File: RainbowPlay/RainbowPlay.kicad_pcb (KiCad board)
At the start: 2 copper layers, 140 x 80 mm, 23 parts, among them J1 GPIO_CONNECTOR, J2 PJ-102A, U1 LM386, U2 LM386

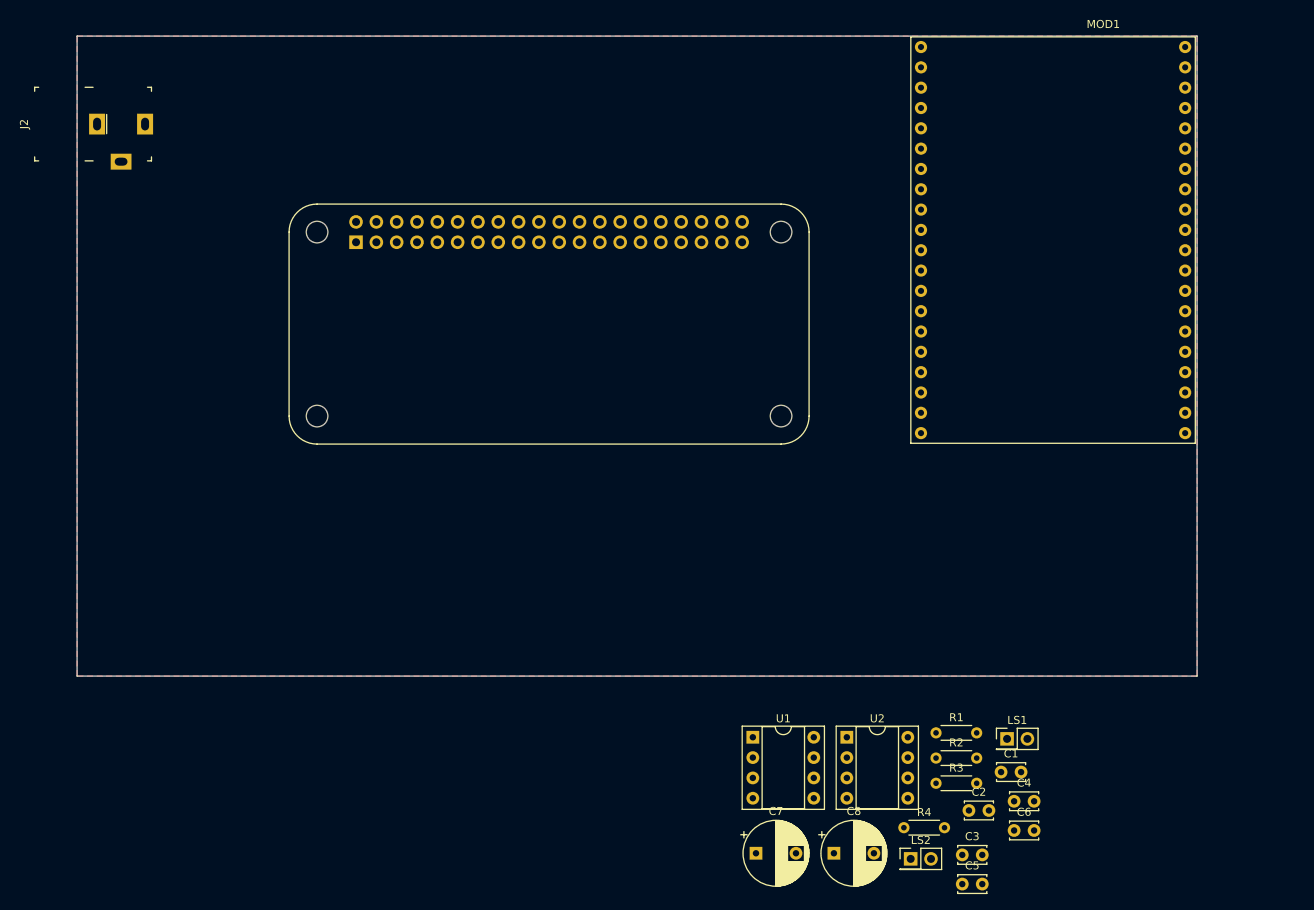
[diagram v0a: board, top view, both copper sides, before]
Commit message: Initial development in progress
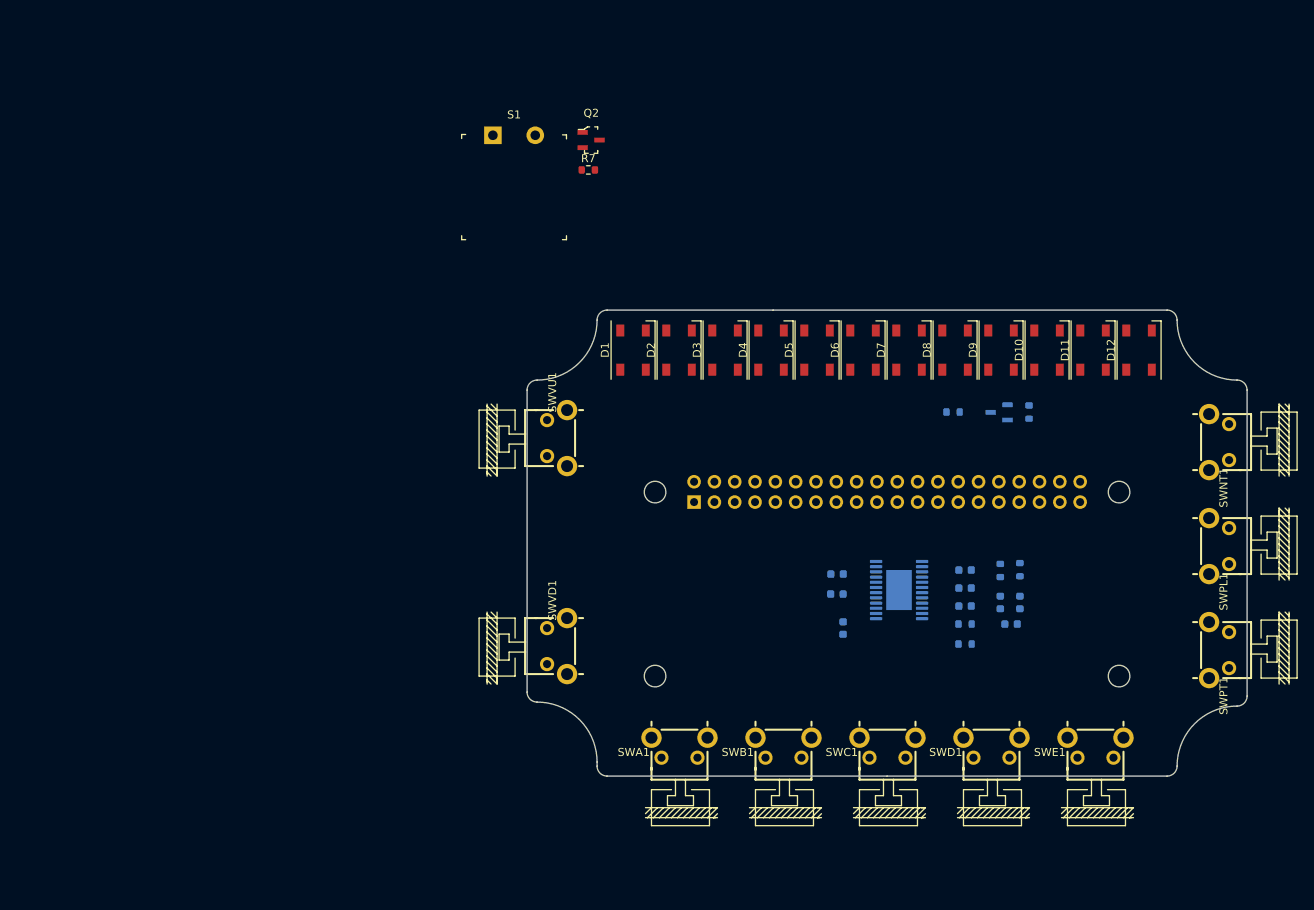
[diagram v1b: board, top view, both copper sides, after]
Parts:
- removed C8: 250uF, Capacitor_THT:CP_Radial_D8.0mm_P5.00mm
- removed J2: PJ-102A, digikey-footprints:Barrel_Jack_5.5mmODx2.1mmID_PJ-102A
- removed LS1, LS2: Speaker, Connector_PinHeader_2.54mm:PinHeader_2x01_P2.54mm_Vertical
- removed MOD1: RN52-I_RM, kicad-footprints:rn52-breakout
- removed U2: LM386, Package_DIP:DIP-8_W7.62mm_Socket
- added D1: SK6812, LED_SMD:LED_SK6812_PLCC4_5.0x5.0mm_P3.2mm, F.Cu at (125.5, 68.8)
- added D10: SK6812, LED_SMD:LED_SK6812_PLCC4_5.0x5.0mm_P3.2mm, F.Cu at (177.3, 68.8)
- added D11: SK6812, LED_SMD:LED_SK6812_PLCC4_5.0x5.0mm_P3.2mm, F.Cu at (183.0, 68.8)
- added D12: SK6812, LED_SMD:LED_SK6812_PLCC4_5.0x5.0mm_P3.2mm, F.Cu at (188.8, 68.8)
- added D2: SK6812, LED_SMD:LED_SK6812_PLCC4_5.0x5.0mm_P3.2mm, F.Cu at (131.3, 68.8)
- added D3: SK6812, LED_SMD:LED_SK6812_PLCC4_5.0x5.0mm_P3.2mm, F.Cu at (137.0, 68.8)
- added D4: SK6812, LED_SMD:LED_SK6812_PLCC4_5.0x5.0mm_P3.2mm, F.Cu at (142.8, 68.8)
- added D5: SK6812, LED_SMD:LED_SK6812_PLCC4_5.0x5.0mm_P3.2mm, F.Cu at (148.5, 68.8)
- added D6: SK6812, LED_SMD:LED_SK6812_PLCC4_5.0x5.0mm_P3.2mm, F.Cu at (154.3, 68.8)
- added D7: SK6812, LED_SMD:LED_SK6812_PLCC4_5.0x5.0mm_P3.2mm, F.Cu at (160.0, 68.8)
- added D8: SK6812, LED_SMD:LED_SK6812_PLCC4_5.0x5.0mm_P3.2mm, F.Cu at (165.8, 68.8)
- added D9: SK6812, LED_SMD:LED_SK6812_PLCC4_5.0x5.0mm_P3.2mm, F.Cu at (171.5, 68.8)
- added L1: 10uH, Inductor_SMD:L_0603_1608Metric, B.Cu at (173.9, 100.4)
- added L2: 10uH, Inductor_SMD:L_0603_1608Metric, B.Cu at (171.4, 100.4)
- added Q1: BSS138, digikey-footprints:SOT-23-3, B.Cu at (171.3, 76.6)
- added Q2: BSS138, digikey-footprints:SOT-23-3, F.Cu at (120.3, 42.6)
- added R5: 10k, Resistor_SMD:R_0603_1608Metric, B.Cu at (175.0, 76.6)
- added R6: 10k, Resistor_SMD:R_0603_1608Metric, B.Cu at (165.5, 76.6)
- added R7: 330, Resistor_SMD:R_0603_1608Metric, F.Cu at (119.9, 46.3)
- added S1: GPTS203211B, digikey-footprints:PushButton_12x12mm_THT_GPTS203211B, F.Cu at (108.0, 42.0)
- added SWA1: B3F-3152, B3F-3152:B3F3152, F.Cu at (127.8, 117.3)
- added SWB1: B3F-3152, B3F-3152:B3F3152, F.Cu at (140.8, 117.3)
- added SWC1: B3F-3152, B3F-3152:B3F3152, F.Cu at (153.8, 117.3)
- added SWD1: B3F-3152, B3F-3152:B3F3152, F.Cu at (166.8, 117.3)
- added SWE1: B3F-3152, B3F-3152:B3F3152, F.Cu at (179.8, 117.3)
- added SWNT1: B3F-3152, B3F-3152:B3F3152, F.Cu at (197.5, 83.8)
- added SWPL1: B3F-3152, B3F-3152:B3F3152, F.Cu at (197.5, 96.8)
- added SWPT1: B3F-3152, B3F-3152:B3F3152, F.Cu at (197.5, 109.8)
- added SWVD1: B3F-3152, B3F-3152:B3F3152, F.Cu at (117.3, 102.3)
- added SWVU1: B3F-3152, B3F-3152:B3F3152, F.Cu at (117.3, 76.3)
- C1, C2: value 10uF -> 1.5uF; footprint Capacitor_THT:C_Disc_D3.4mm_W2.1mm_P2.50mm -> Capacitor_SMD:C_0603_1608Metric; moved to B.Cu
- C3: value 0.1uF -> 1uF; footprint Capacitor_THT:C_Disc_D3.4mm_W2.1mm_P2.50mm -> Capacitor_SMD:C_0603_1608Metric; moved to B.Cu
- C4: value 0.1uF -> 47nF; footprint Capacitor_THT:C_Disc_D3.4mm_W2.1mm_P2.50mm -> Capacitor_SMD:C_0603_1608Metric; moved to B.Cu
- C5, C6: value 0.05uF -> 47nF; footprint Capacitor_THT:C_Disc_D3.4mm_W2.1mm_P2.50mm -> Capacitor_SMD:C_0603_1608Metric; moved to B.Cu
- C7: value 250uF -> 47nF; footprint Capacitor_THT:CP_Radial_D8.0mm_P5.00mm -> Capacitor_SMD:C_0603_1608Metric; moved to B.Cu
- H1, H2, H3, H4: moved to B.Cu
- R1, R2: value 1.2k -> 5R; footprint Resistor_THT:R_Axial_DIN0204_L3.6mm_D1.6mm_P5.08mm_Horizontal -> Resistor_SMD:R_0603_1608Metric; moved to B.Cu
- R3, R4: value 10R -> 2.2k; footprint Resistor_THT:R_Axial_DIN0204_L3.6mm_D1.6mm_P5.08mm_Horizontal -> Resistor_SMD:R_0603_1608Metric; moved to B.Cu
- U1: value LM386 -> TPA2001D2; footprint Package_DIP:DIP-8_W7.62mm_Socket -> Package_SO:HTSSOP-24-1EP_4.4x7.8mm_P0.65mm_EP3.2x5mm; moved to B.Cu
- moved H1 105.4 mm to (186.3, 86.6), turned to 180 degrees
- moved H4 105.4 mm to (186.3, 109.6), turned to 180 degrees
- moved J1 53.3 mm to (133.2, 87.8)
- moved C5 37.0 mm to (167.0, 98.6), turned to 180 degrees
- moved C7 36.3 mm to (151.0, 96.8), turned to 180 degrees
- moved H2 36.1 mm to (128.3, 86.6), turned to 180 degrees
- moved H3 36.1 mm to (128.3, 109.6), turned to 180 degrees
- moved C6 33.1 mm to (151.8, 103.6), turned to 270 degrees
- moved C3 31.1 mm to (167.0, 100.8), turned to 180 degrees
- moved C1 30.3 mm to (151.0, 99.3)
- moved C4 29.5 mm to (167.0, 96.3), turned to 180 degrees
- moved U1 25.9 mm to (158.8, 98.8)
- moved R2 24.8 mm to (171.4, 96.4), turned to 90 degrees
- moved R4 24.2 mm to (167.0, 105.6)
- moved C2 23.9 mm to (172.8, 103.1)
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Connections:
- C1 pad 2: Net-(C1-Pad2) -> GNDA
- C2 pad 2: Net-(C2-Pad2) -> Net-(C1-Pad1)
- C3 pad 1: GNDA -> /MIC_BIAS
- C3 pad 2: Net-(C3-Pad2) -> GNDA
- C4 pad 1: GNDA -> /MIC_BIAS
- C4 pad 2: Net-(C4-Pad2) -> /MIC_R+
- C5 pad 1: Net-(C5-Pad1) -> /MIC_BIAS
- C5 pad 2: GNDA -> /MIC_L+
- C6 pad 1: Net-(C6-Pad1) -> /MIC_L-
- C6 pad 2: GNDA -> Net-(C2-Pad1)
- C7 pad 1: Net-(C7-Pad1) -> /MIC_R-
- C7 pad 2: Net-(C7-Pad2) -> Net-(C1-Pad1)
- J1 pad 10: /GPIO15_RXD0 -> (no net)
- J1 pad 12: (no net) -> /LED
- J1 pad 16: (no net) -> /BTN_A
- J1 pad 17: +3V3 -> (no net)
- J1 pad 18: (no net) -> /BTN_B
- J1 pad 2: +15V -> +5V
- J1 pad 20: (no net) -> GND
- J1 pad 27: (no net) -> /BTN_C
- J1 pad 29: (no net) -> /BTN_D
- J1 pad 31: (no net) -> /BTN_E
- J1 pad 32: (no net) -> /PWM_AUDIO_L
- J1 pad 33: (no net) -> /PWM_AUDIO_R
- J1 pad 39: GND -> (no net)
- J1 pad 4: +15V -> +5V
- J1 pad 40: (no net) -> /PWR_BTN
- J1 pad 8: /GPIO14_TXD0 -> (no net)
- R1 pad 1: Net-(R1-Pad1) -> Net-(L1-Pad1)
- R1 pad 2: Net-(C1-Pad2) -> /PWM_AUDIO_R
- R2 pad 2: Net-(C2-Pad2) -> /PWM_AUDIO_L
- R3 pad 1: Net-(C7-Pad1) -> Net-(C1-Pad1)
- R3 pad 2: Net-(C5-Pad1) -> /MIC_BIAS
- R4 pad 1: Net-(C8-Pad1) -> Net-(C2-Pad1)
- R4 pad 2: Net-(C6-Pad1) -> /MIC_BIAS
- U1 pad 1: Net-(R1-Pad1) -> GNDPWR
- U1 pad 2: /SPK_R- -> (no net)
- U1 pad 3: /SPK_R+ -> (no net)
- U1 pad 4: GNDA -> (no net)
- U1 pad 5: Net-(C7-Pad1) -> /MIC_L-
- U1 pad 6: +15V -> GNDA
- U1 pad 7: Net-(C3-Pad2) -> (no net)
- U1 pad 8: Net-(C1-Pad1) -> /MIC_R-
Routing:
- added copper zone on In2.Cu, net GND
- removed copper zone on F.Cu, net GND
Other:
- board size 140 x 80 mm -> 90 x 58.2 mm
- copper layers 2 -> 4
- board text removed: "Board Corner Radius = 3mm All holes are M2.5"
